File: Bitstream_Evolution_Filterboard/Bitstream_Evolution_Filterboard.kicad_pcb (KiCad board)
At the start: 2 copper layers, 65.8 x 35.8 mm, 7 parts, among them J1 Conn_01x15_Female, J2 Conn_01x15_Female, J3 Conn_01x10_Female, J4 Conn_01x10_Female, J5 Conn_01x02_Male

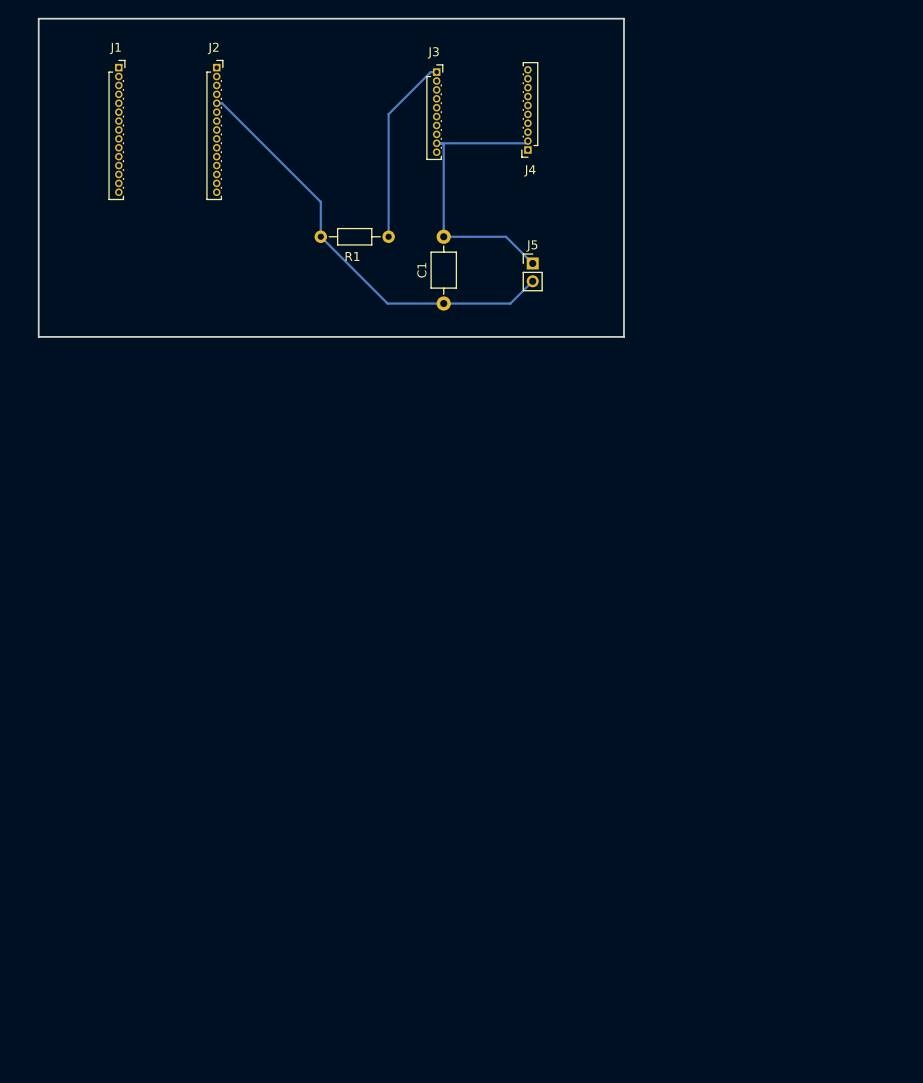
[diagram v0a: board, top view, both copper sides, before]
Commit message: Updates to Hardware
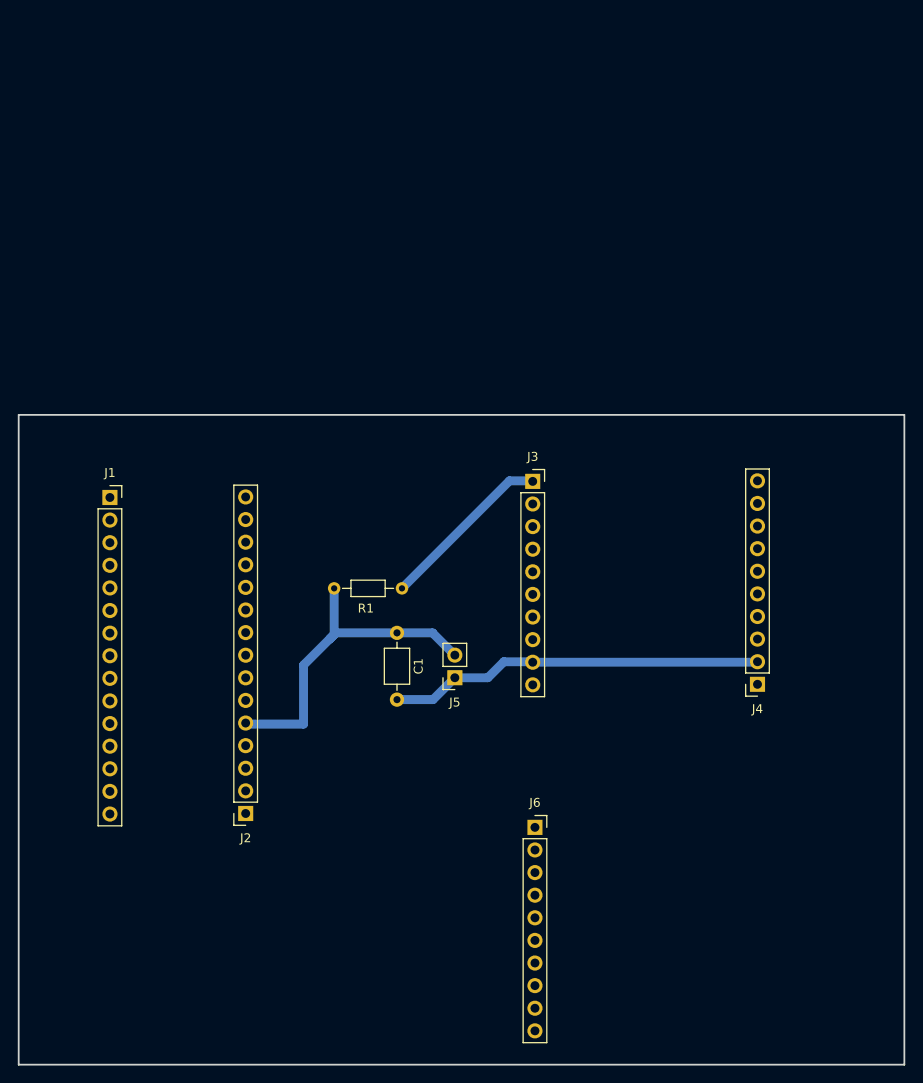
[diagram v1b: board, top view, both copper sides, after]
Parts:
- added J6: Conn_01x10_Female, Connector_PinSocket_2.54mm:PinSocket_1x10_P2.54mm_Vertical, F.Cu at (139.2, 135.6)
- J1, J2: footprint Connector_PinSocket_1.00mm:PinSocket_1x15_P1.00mm_Vertical -> Connector_PinSocket_2.54mm:PinSocket_1x15_P2.54mm_Vertical
- J3, J4: footprint Connector_PinSocket_1.00mm:PinSocket_1x10_P1.00mm_Vertical -> Connector_PinSocket_2.54mm:PinSocket_1x10_P2.54mm_Vertical
- J5: footprint Connector_PinHeader_2.00mm:PinHeader_1x02_P2.00mm_Vertical -> Connector_PinSocket_2.54mm:PinSocket_1x02_P2.54mm_Vertical
- moved J2 83.9 mm to (106.8, 134.0), turned to 180 degrees
- moved J4 65.3 mm to (164.2, 119.5)
- moved J1 48.3 mm to (91.5, 98.5)
- moved J5 47.4 mm to (130.2, 118.8), turned to 180 degrees
- moved J3 47.2 mm to (139.0, 96.7)
- moved R1 39.5 mm to (124.3, 108.8)
- moved C1 37.4 mm to (123.8, 113.8), turned to -90 degrees
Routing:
- net /Output: track 48.1 -> 38.6 mm
- net GND: track 32.8 -> 42.3 mm
- net /Input: track 21.5 -> 19.7 mm
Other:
- board size 65.8 x 35.8 mm -> 99.5 x 73 mm
